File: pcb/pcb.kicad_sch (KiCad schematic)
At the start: 12 parts, among them J1 GND, J2 HC-SR04, J3 PWM, J4 GPS UART, J5 Power Module v1.0, J6 UART, SW1 Reset, SW2 Action, U1 Pico, U2 NRF24L01, U3 MPU9250, U4 BMP280

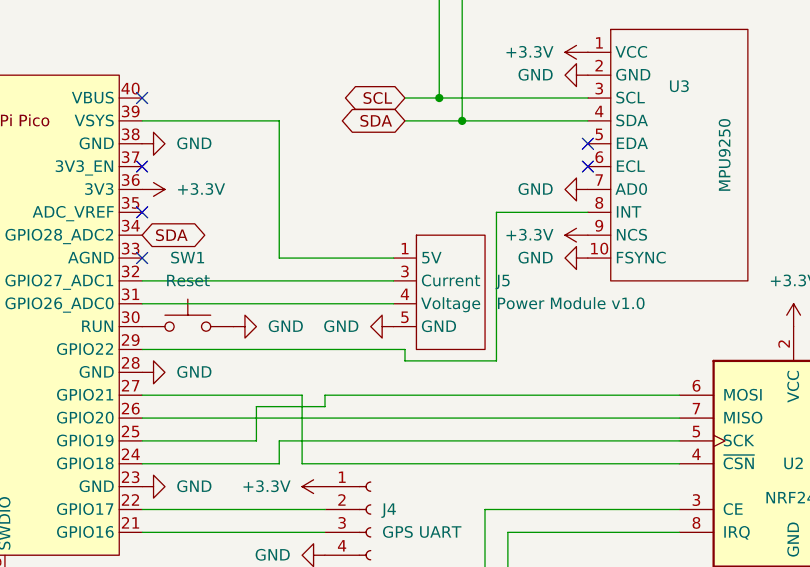
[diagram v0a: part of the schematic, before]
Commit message: More sweeping changes, soon IO will be done?
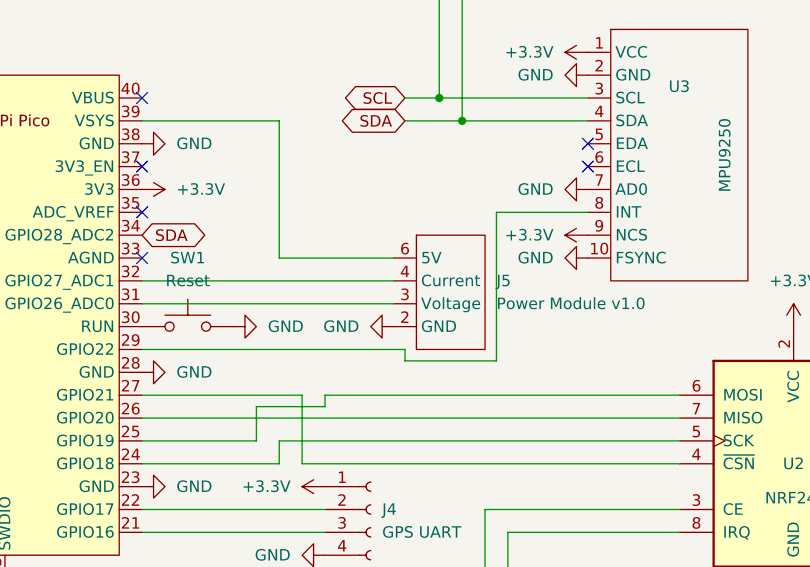
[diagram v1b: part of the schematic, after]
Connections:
- net GND: now also J5.1 (GND), J5.2 (GND); no longer J5.5 (GND), J5.6 (GND)
- net at J5.3 (Voltage): now also U1.31 (GPIO26_ADC0); no longer U1.32 (GPIO27_ADC1)
- net at J5.4 (Current): now also U1.32 (GPIO27_ADC1); no longer U1.31 (GPIO26_ADC0)
- new net: J5.5 (5V), J5.6 (5V), U1.39 (VSYS)

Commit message: Refactored organization
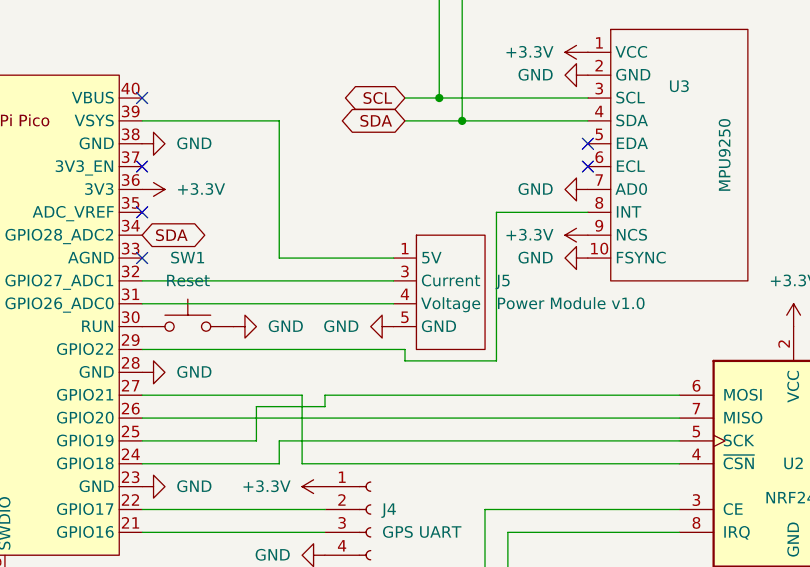
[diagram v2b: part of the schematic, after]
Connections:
- net GND: now also J5.5 (GND), J5.6 (GND); no longer J5.1 (GND), J5.2 (GND)
- net at J5.3 (Current): now also U1.32 (GPIO27_ADC1); no longer U1.31 (GPIO26_ADC0)
- net at J5.4 (Voltage): now also U1.31 (GPIO26_ADC0); no longer U1.32 (GPIO27_ADC1)
- new net: J5.1 (5V), J5.2 (5V), U1.39 (VSYS)
